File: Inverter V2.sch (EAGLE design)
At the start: 30 parts, among them Q1 ROHM_SCT3022ALGC11ROHM_SCT302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, Q2 ROHM_SCT3022ALGC11ROHM_SCT302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, Q3 ROHM_SCT3022ALGC11ROHM_SCT302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, Q4 ROHM_SCT3022ALGC11ROHM_SCT302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, Q5 ROHM_SCT3022ALGC11ROHM_SCT302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, Q6 ROHM_SCT3022ALGC11ROHM_SCT302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, U1 RASPBERRY_PICOTH

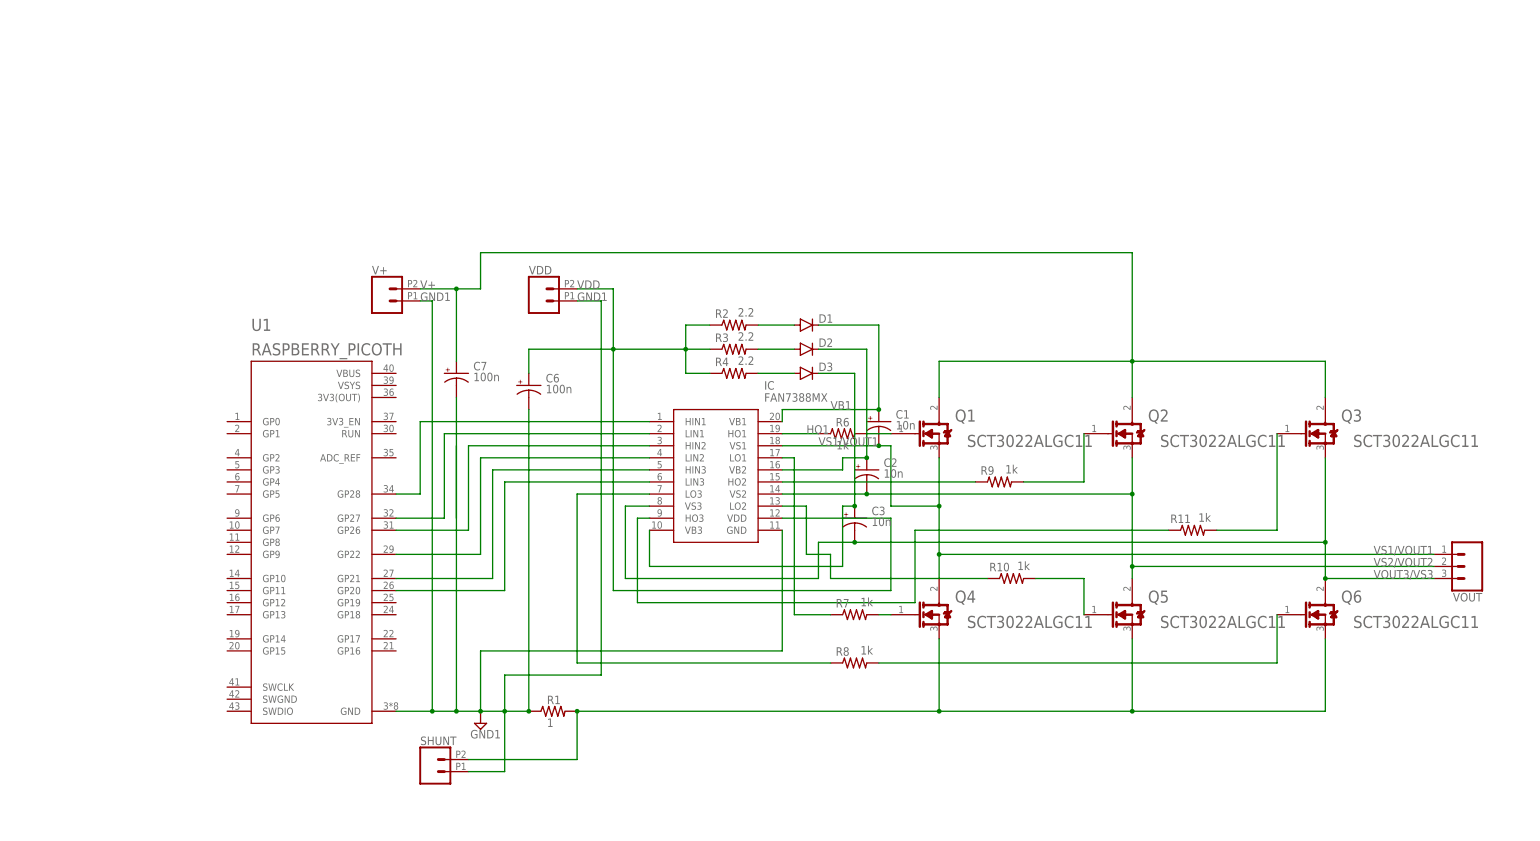
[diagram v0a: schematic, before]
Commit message: Routing Inverter V2
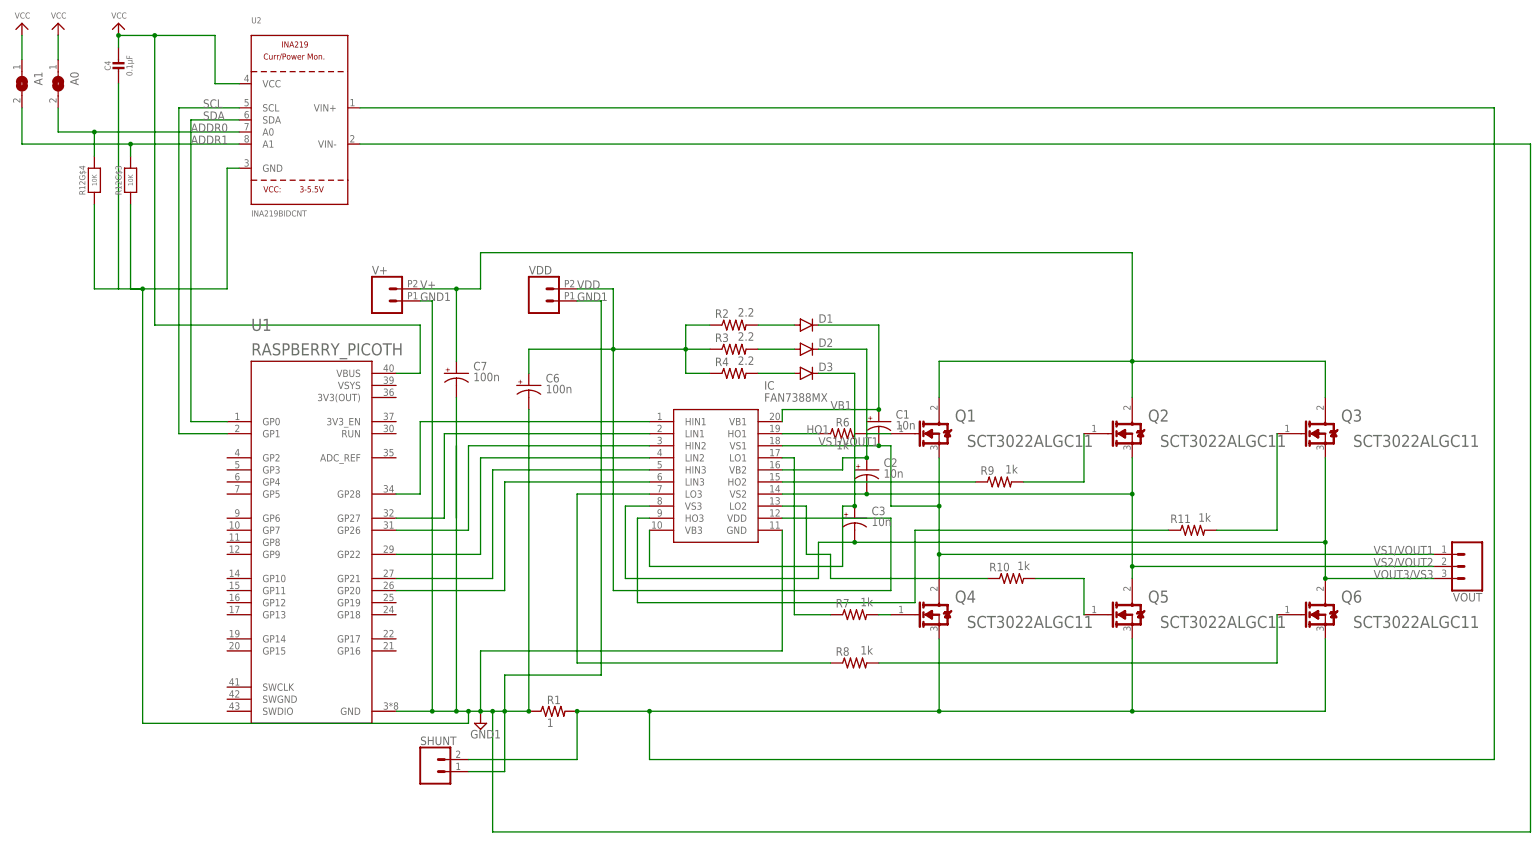
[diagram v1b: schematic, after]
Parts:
- added A0, A1: (no value), microbuilder:SOLDERJUMPERREFLOW_NOPASTE
- added C4: 0.1µF, microbuilder:CAP_CERAMIC0603_NO
- added R12: 10K, microbuilder:RESISTOR_4PACK
- added U2: INA219BIDCNT, microbuilder:INA219
- SHUNT: device SparkFun-Connectors:CONN_022.54MM_SCREWTERM -> SparkFun-Connectors:CONN_02PTH4
- VOUT: device SparkFun-Connectors:CONN_03SCREW_LOCK -> SparkFun-Connectors:CONN_03SCREW-NS
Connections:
- net N$1 renamed HIN1
- net N$10 renamed VGIN3
- net N$11 renamed VGIN2
- net N$12 renamed HO3
- net N$14 renamed VGIN6
- net N$16 renamed VGIN4
- net N$2 renamed LO1
- net N$3 renamed LIN1
- net N$5 renamed LIN2
- net N$6 renamed VGIN1
- net N$7 renamed HIN3
- net N$8 renamed VGIN5
- net N$9 renamed LIN3
- new net ADDR0: A0.2, R12G$4.2, U2.A0
- new net ADDR1: A1.2, R12G$3.2, U2.A1
- new net SCL: U1.GP1, U2.SCL
- new net SDA: U1.GP0, U2.SDA
- new net VCC: A0.1, A1.1, C4.1, U1.VBUS, U2.VCC
- net GND1: now also C4.2, R12G$3.1, R12G$4.1, U2.GND, U2.VIN-
- net SHUNT: now also U2.VIN+

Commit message: Revision to routed V2 inverter
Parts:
- C7: device rcl:CPOL-USSMCZ -> rcl:CPOL-USE5-5
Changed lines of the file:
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@@
 <part name="C1" library="rcl" library_urn="urn:adsk.eagle:library:334" deviceset="CPOL-US" device="SMCZ" package3d_urn="urn:adsk.eagle:package:25927/3" value="10n"/>
 <part name="C2" library="rcl" library_urn="urn:adsk.eagle:library:334" deviceset="CPOL-US" device="SMCZ" package3d_urn="urn:adsk.eagle:package:25927/3" value="10n"/>
-<part name="C7" library="rcl" library_urn="urn:adsk.eagle:library:334" deviceset="CPOL-US" device="SMCZ" package3d_urn="urn:adsk.eagle:package:25927/3" value="100n"/>
+<part name="C7" library="rcl" library_urn="urn:adsk.eagle:library:334" deviceset="CPOL-US" device="E5-5" package3d_urn="urn:adsk.eagle:package:23367/2" value="100n"/>
 <part name="V+" library="SparkFun-Connectors" deviceset="CONN_02" device="2.54MM_SCREWTERM"/>
 <part name="VDD" library="SparkFun-Connectors" deviceset="CONN_02" device="2.54MM_SCREWTERM"/>
